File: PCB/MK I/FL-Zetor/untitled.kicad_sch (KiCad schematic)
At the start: 16 parts, among them J1 Conn_01x02_Pin, J2 Conn_01x06_Pin, J3 Conn_01x06_Pin, J4 Conn_01x06_Pin, J5 Conn_01x06_Pin, SW1 SL19, U1 TSOP382xx, U2 LM1086

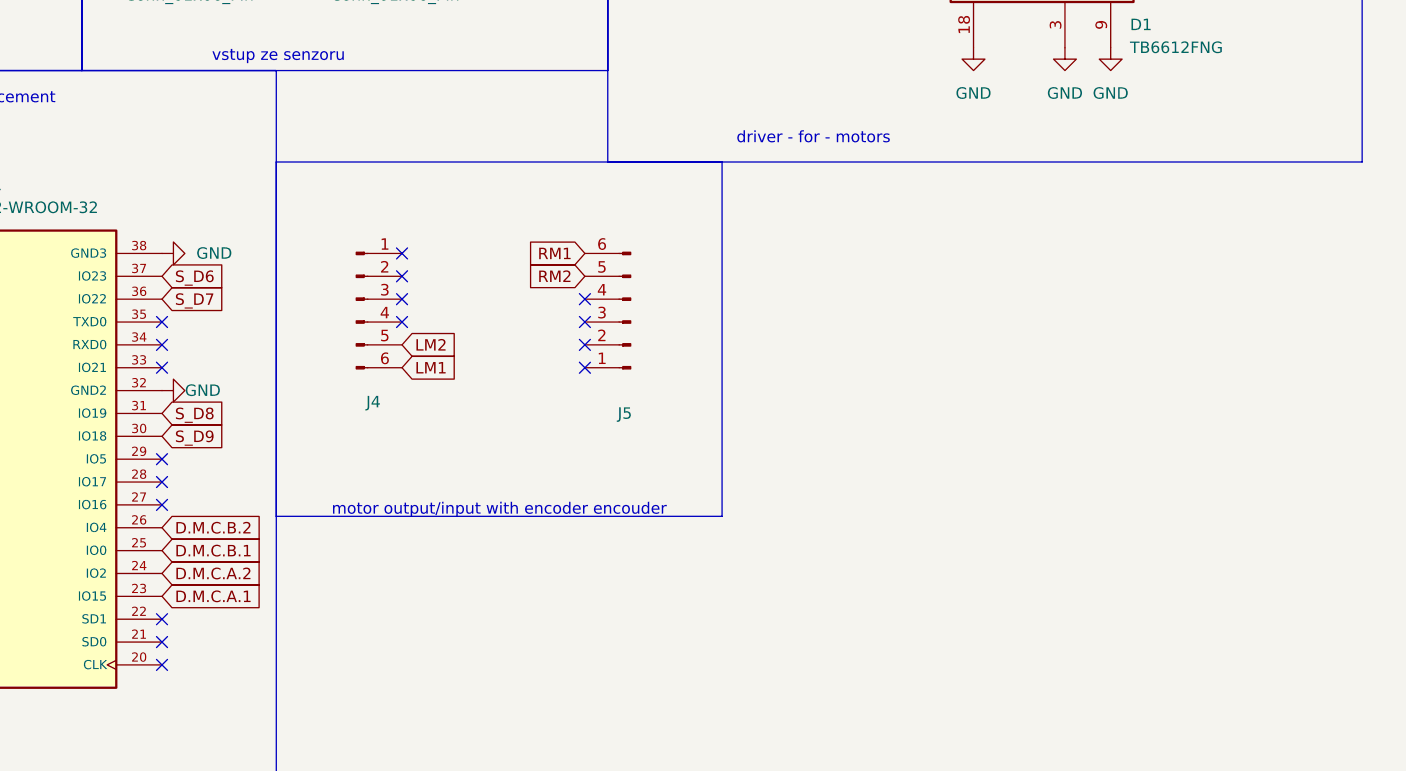
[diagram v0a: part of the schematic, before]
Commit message: pcbs done
that pieces of craps is done
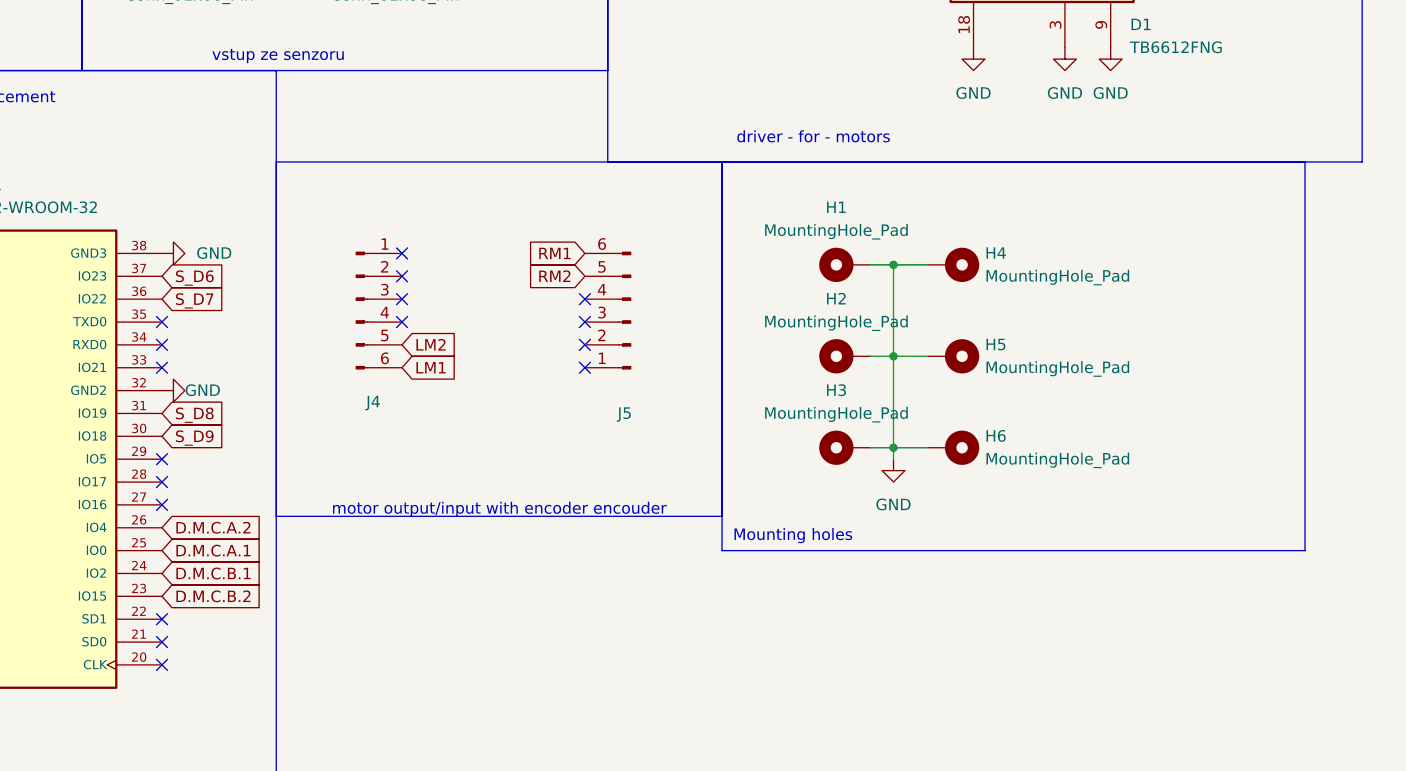
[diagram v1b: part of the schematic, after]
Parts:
- added H1, H2, H3, H4, H5, H6: MountingHole_Pad, MountingHole:MountingHole_3.2mm_M3_ISO7380_Pad, symbol Mechanical:MountingHole_Pad
- C3, C5: footprint Capacitor_Tantalum_SMD:CP_EIA-7343-31_Kemet-D -> Capacitor_SMD:C_0805_2012Metric_Pad1.18x1.45mm_HandSolder
- J1: footprint Connector_AMASS:AMASS_XT30PW-M_1x02_P2.50mm_Horizontal -> Connector_AMASS:AMASS_XT30U-F_1x02_P5.0mm_Vertical
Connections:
- net D.M.C.A.1: now also MCU1.25 (IO0); no longer MCU1.23 (IO15)
- net D.M.C.A.2: now also MCU1.26 (IO4); no longer MCU1.24 (IO2)
- net D.M.C.B.1: now also MCU1.24 (IO2); no longer MCU1.25 (IO0)
- net D.M.C.B.2: now also MCU1.23 (IO15); no longer MCU1.26 (IO4)
- net GND: now also H1.1, H2.1, H3.1, H4.1, H5.1, H6.1
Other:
- note added: "Mounting holes"
